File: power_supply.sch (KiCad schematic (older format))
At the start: 68 parts, among them J1 USB-MICRO, J2 USB, Q1 SI4174DY, Q2 SI4463CDY, Q3 SW, U1 LM3914, U10 LT1494, U2 TPD2E001DRL, U3 MIC2185, U4 TPS2511, U5 MCP73833, U6 TPD2E001DRL, U7 BATT, U8 MAX9938T, U9 FDC6392S

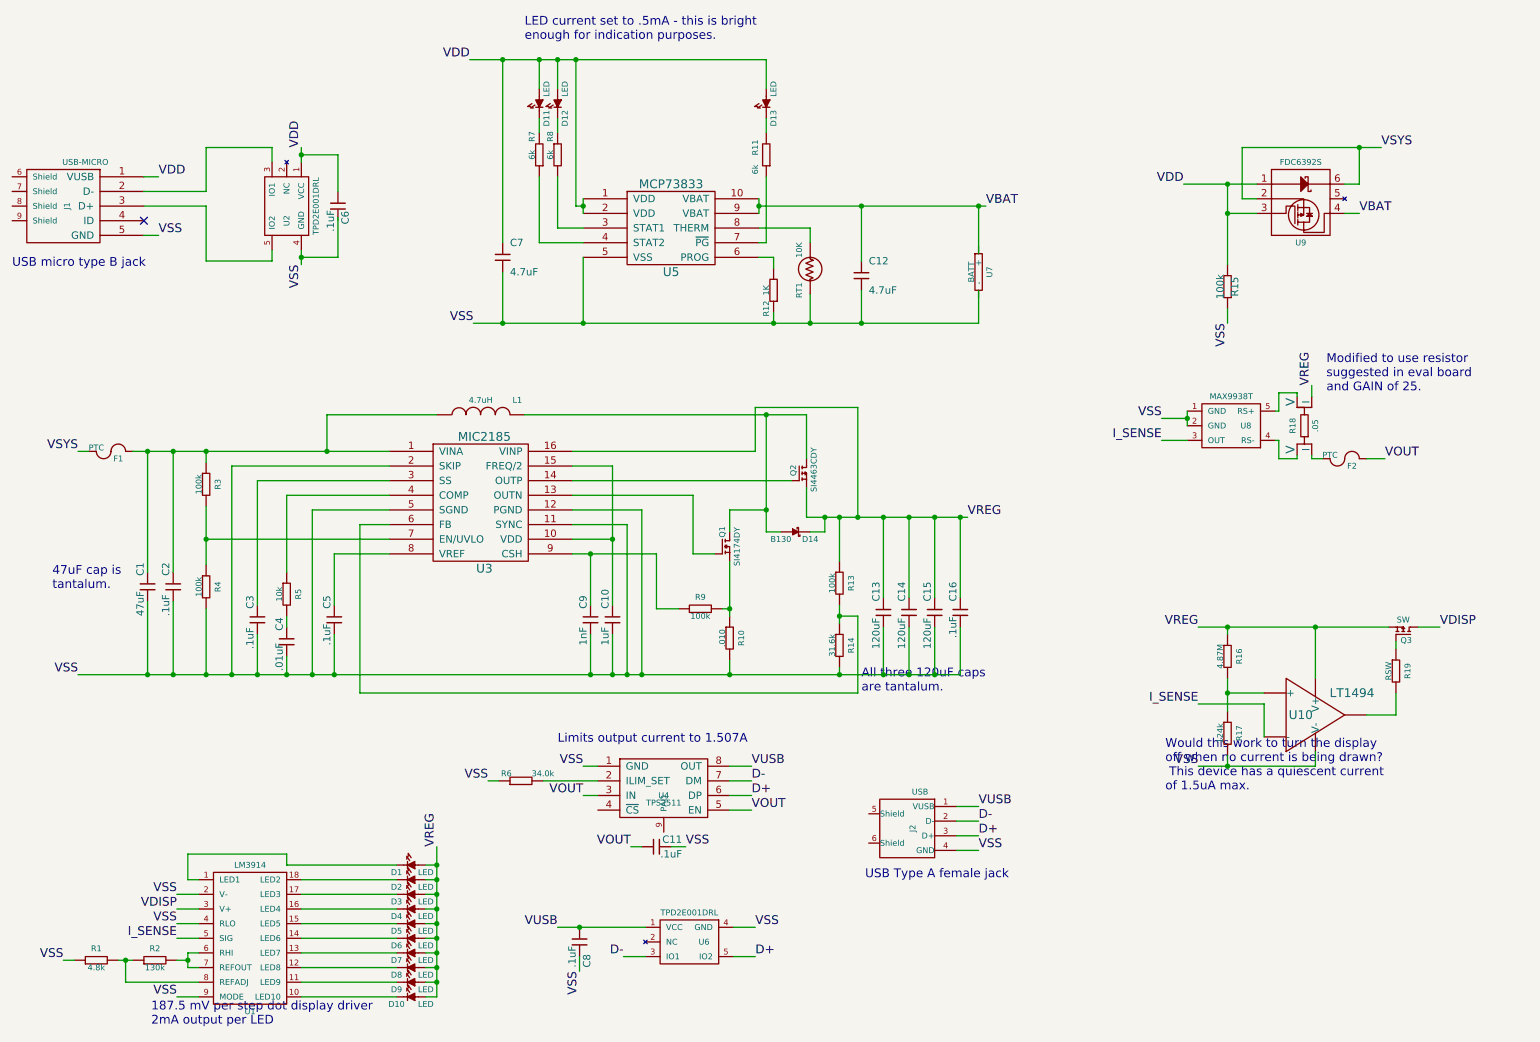
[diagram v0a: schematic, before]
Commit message: Fixed a few issues with printout
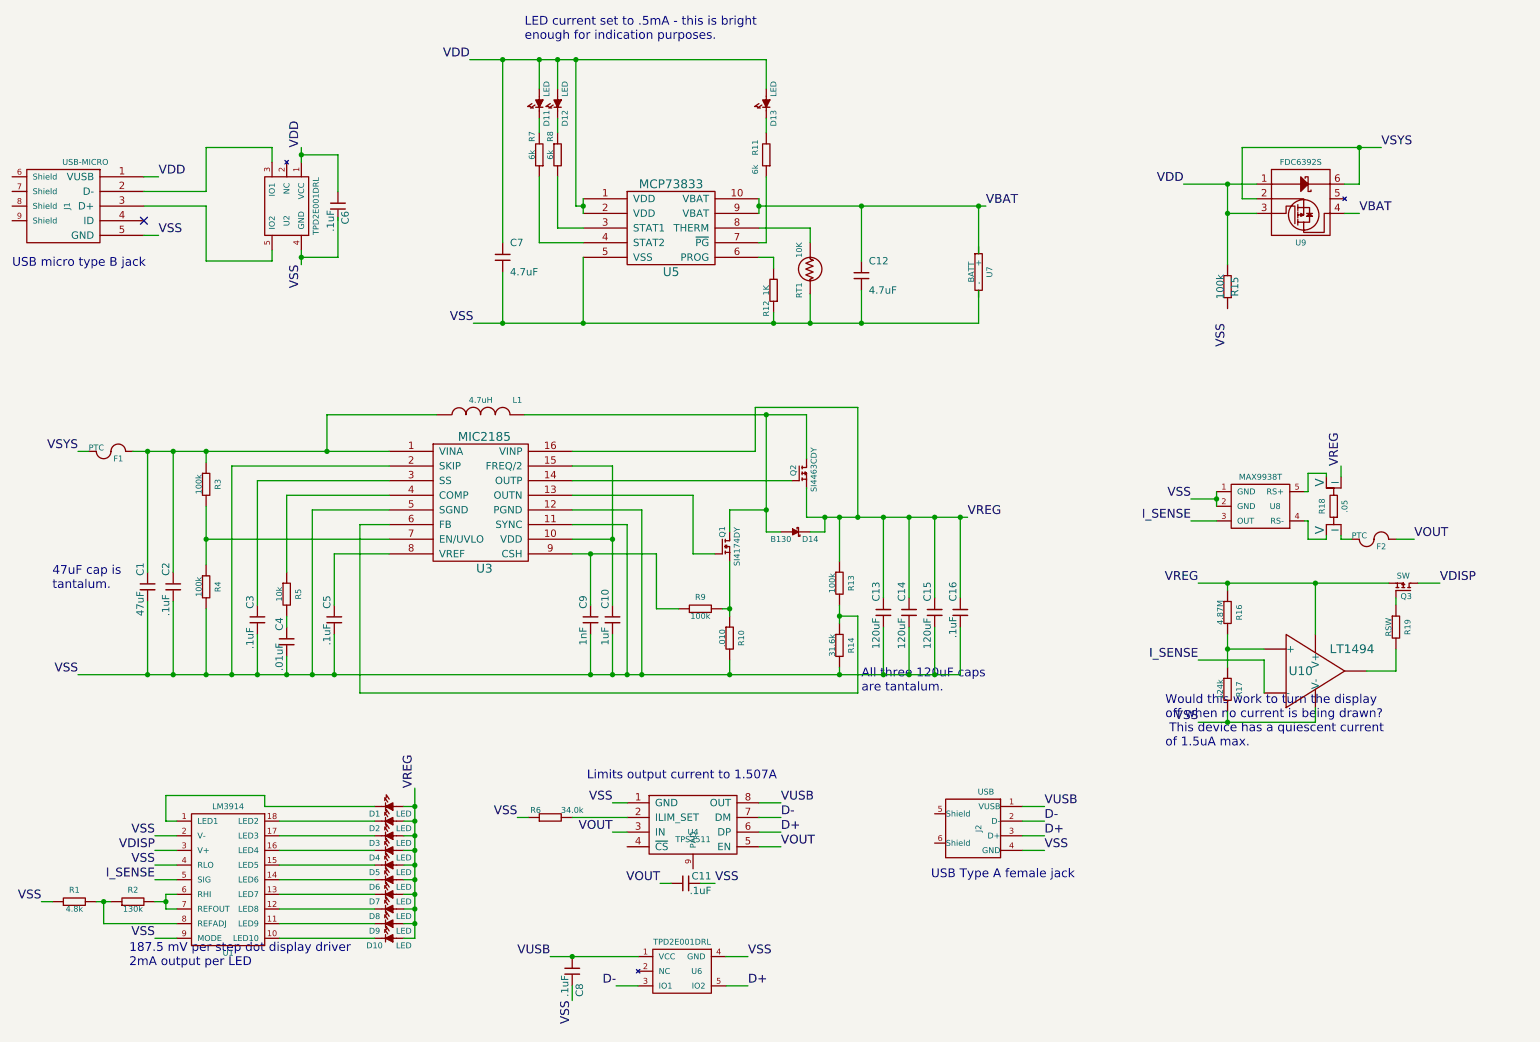
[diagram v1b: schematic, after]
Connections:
- net VSS: no longer R15.1
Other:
- note removed: "Modified to use resistor \nsuggested in eval board \nand GAIN of 25."
- moved on the sheet: C11, C8, D1, D10, D2, D3, D4, D5, D6, D7, D8, D9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
